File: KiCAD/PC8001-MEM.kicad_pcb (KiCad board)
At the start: 2 copper layers, 100 x 75 mm, 33 parts, among them J1 PC-8001 ext BUS, U1 74LS32, U10 628128, U2 74LS138, U3 ULN2003A, U4 74LS138, U5 74LS175, U6 74LS32, U7 74LS541, U8 74LS273, U9 74LS541

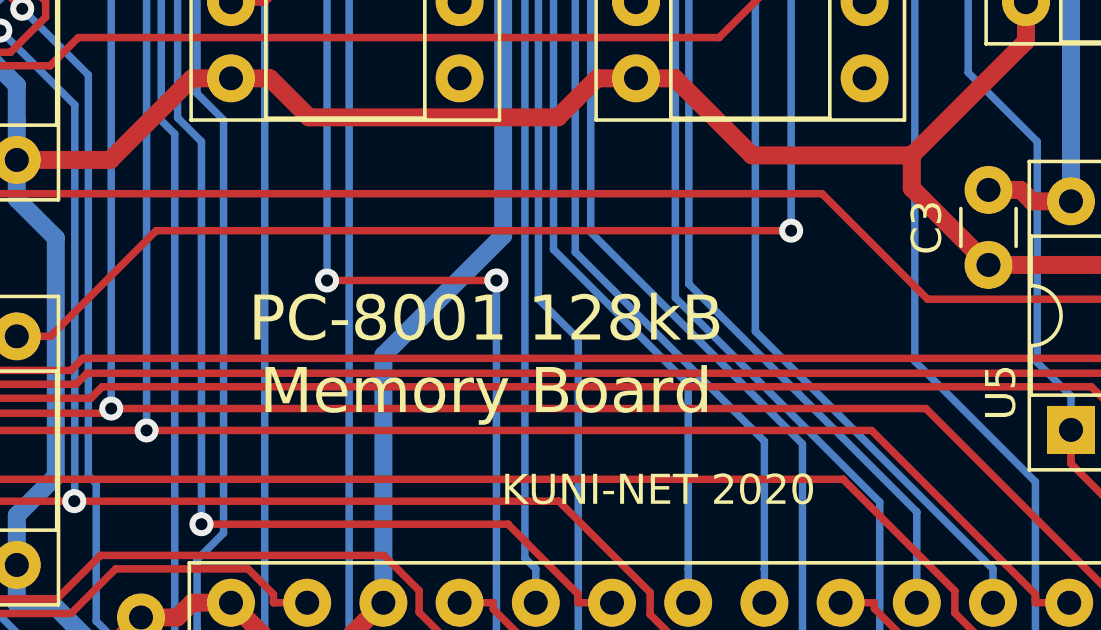
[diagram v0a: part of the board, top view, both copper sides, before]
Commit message: パターン更新
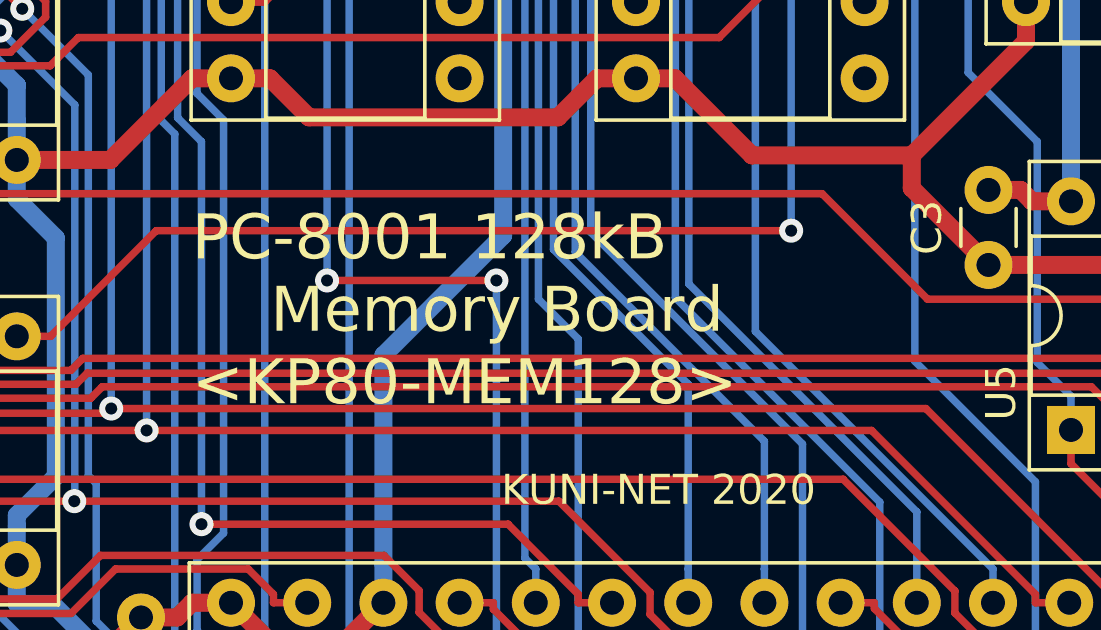
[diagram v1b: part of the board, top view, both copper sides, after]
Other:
- board text added: "PC-8001 128kB Memory Board <KP80-MEM128>"
- board text removed: "PC-8001 128kB Memory Board"
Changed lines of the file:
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@@
     (effects (font (size 1 1) (thickness 0.15)))
   )
-  (gr_text "PC-8001 128kB \nMemory Board" (at 154 100.5) (layer F.SilkS)
-    (effects (font (size 1.5 1.5) (thickness 0.2)))
+  (gr_text "PC-8001 128kB \n    Memory Board\n<KP80-MEM128>" (at 144.2 99) (layer F.SilkS)
+    (effects (font (size 1.5 1.5) (thickness 0.2)) (justify left))
   )
   (gr_text "KUNI-NET 2020" (at 159.75 105) (layer F.SilkS)
